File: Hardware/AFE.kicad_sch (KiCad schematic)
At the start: 29 parts, among them U301 LTC6268IS6, U302 AD8139

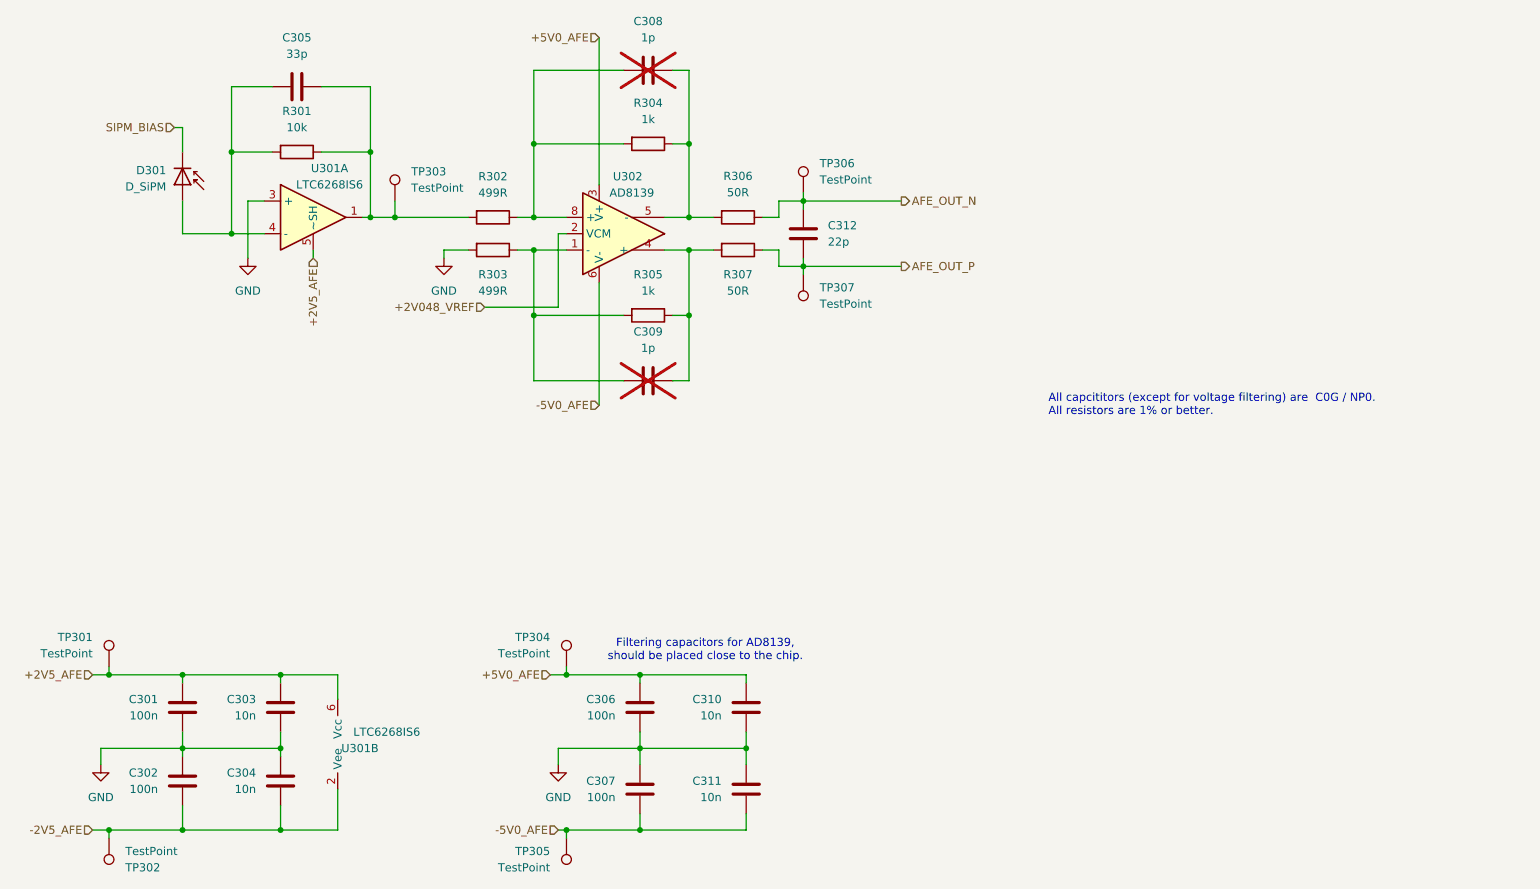
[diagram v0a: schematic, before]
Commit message: fix: #170, fix: #144, fix: #132
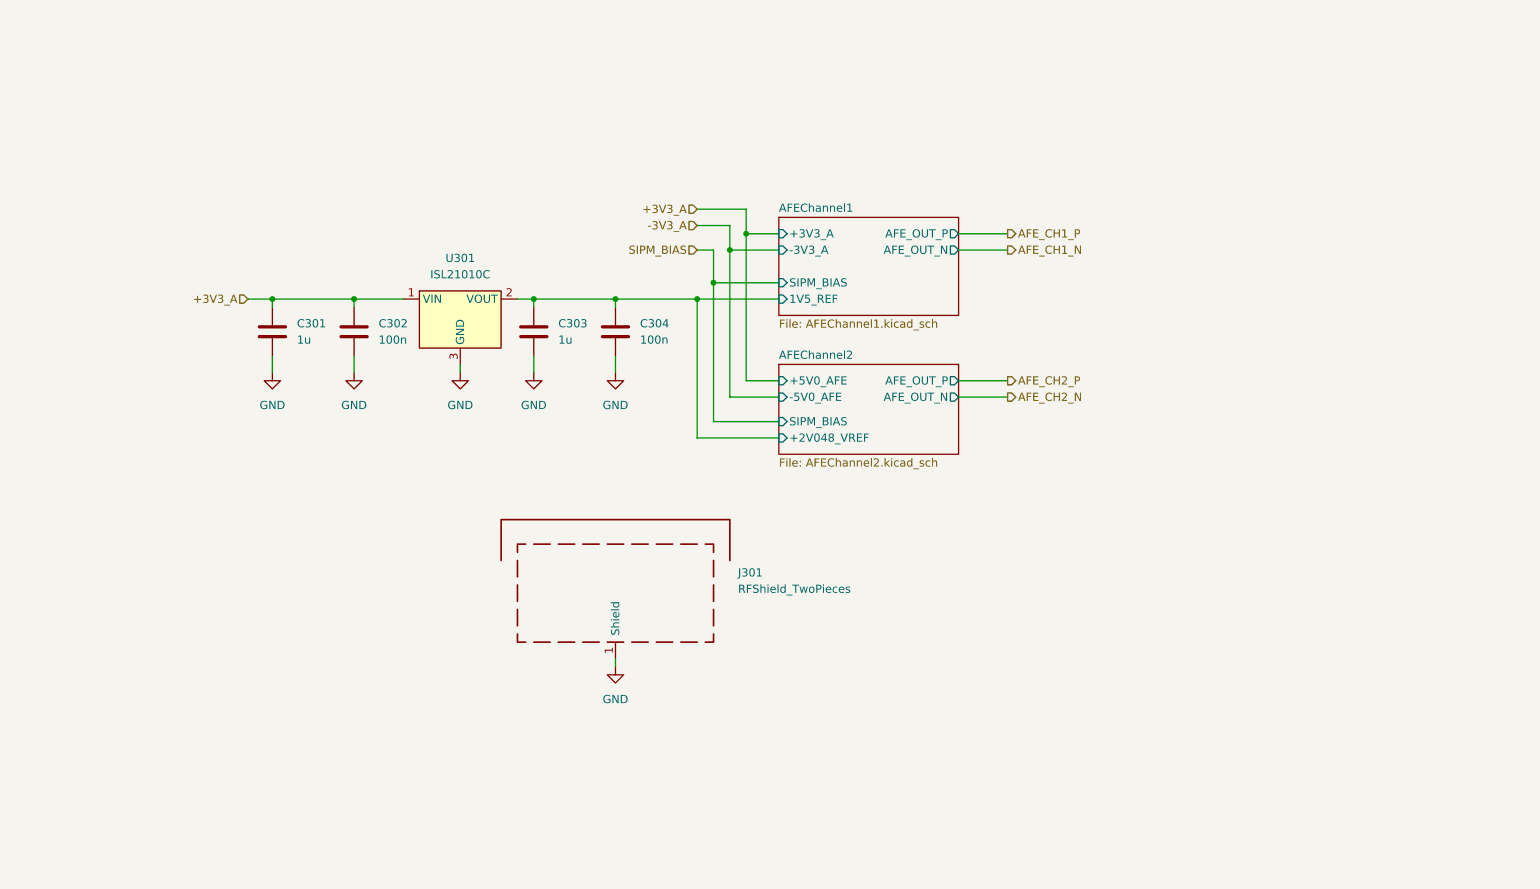
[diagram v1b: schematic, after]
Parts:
- removed C305: 33p, Capacitor_SMD:C_0805_2012Metric, symbol Device:C
- removed C306, C307: 100n, Capacitor_SMD:C_0805_2012Metric, symbol Device:C
- removed C308, C309: 1p, Capacitor_SMD:C_0805_2012Metric, symbol Device:C
- removed C310, C311: 10n, Capacitor_SMD:C_0805_2012Metric, symbol Device:C
- removed C312: 22p, Capacitor_SMD:C_0805_2012Metric, symbol Device:C
- removed D301: D_SiPM, symbol Device:D_SiPM
- removed R301: 10k, Resistor_SMD:R_0805_2012Metric, symbol Device:R
- removed R302, R303: 499R, Resistor_SMD:R_0805_2012Metric, symbol Device:R
- removed R304, R305: 1k, Resistor_SMD:R_0805_2012Metric, symbol Device:R
- removed R306, R307: 50R, Resistor_SMD:R_0805_2012Metric, symbol Device:R
- removed TP301, TP302, TP303, TP304, TP305, TP306, TP307: TestPoint, TestPoint:TestPoint_Pad_D1.5mm, symbol Connector:TestPoint
- removed U301: LTC6268IS6, Package_TO_SOT_SMD:TSOT-23-6_HandSoldering, symbol DataAcquisitionUnit:LTC6268IS6_TSOT-23
- removed U302: AD8139, Package_SO:SOIC-8_5.3x5.3mm_P1.27mm, symbol DataAcquisitionUnit:AD8139
- added J301: RFShield_TwoPieces, GammaSpectrometer:BUD_CU-470_Shield, symbol Device:RFShield_TwoPieces
- added U301: ISL21010C, Package_TO_SOT_SMD:SOT-23, symbol GammaSpectrometer:ISL21010C
- C301: value 100n -> 1u
- C303: value 10n -> 1u
- C304: value 10n -> 100n
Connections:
- net -2V5_AFE is gone; now on net GND: C302.2, C304.2
- net GND: now also J301.1 (Shield), U301.3 (GND); no longer C302.1, C304.1
- net +2V5_AFE renamed +3V3_A
- net +3V3_A: now also C302.1, U301.1 (VIN); no longer C303.1
- new net AFEChannel1/1V5_REF: C303.1, C304.1, U301.2 (VOUT)
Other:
- added sheet AFEChannel1 (AFEChannel1.kicad_sch)
- added sheet AFEChannel2 (AFEChannel2.kicad_sch)
- note removed: "All capcititors (except for voltage filtering) are C0G / NP0. All resistors are 1% or better."
- note removed: "Filtering capacitors for AD8139, should be placed close to the chip."
